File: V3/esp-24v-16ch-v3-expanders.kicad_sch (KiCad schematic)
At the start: 4 parts, among them U6 MCP23017_SS, U7 MCP23017_SS

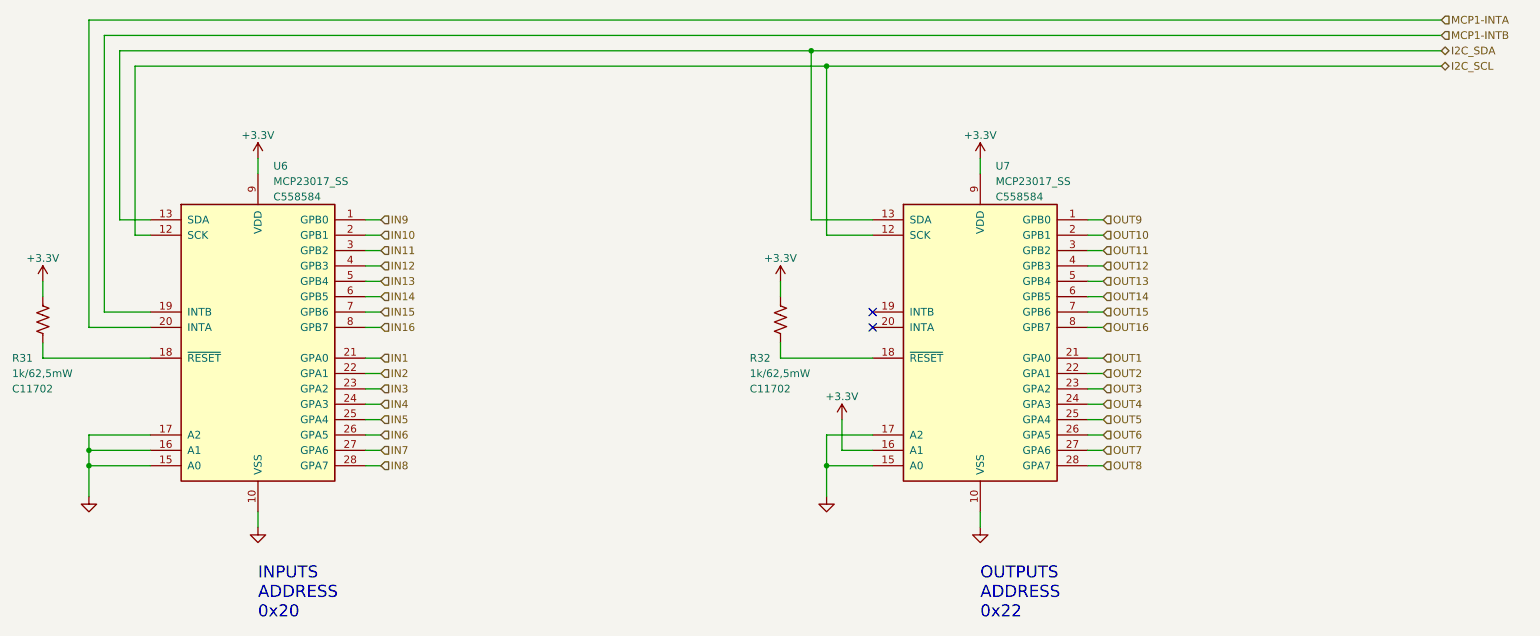
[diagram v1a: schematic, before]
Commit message: Added temperature sensor
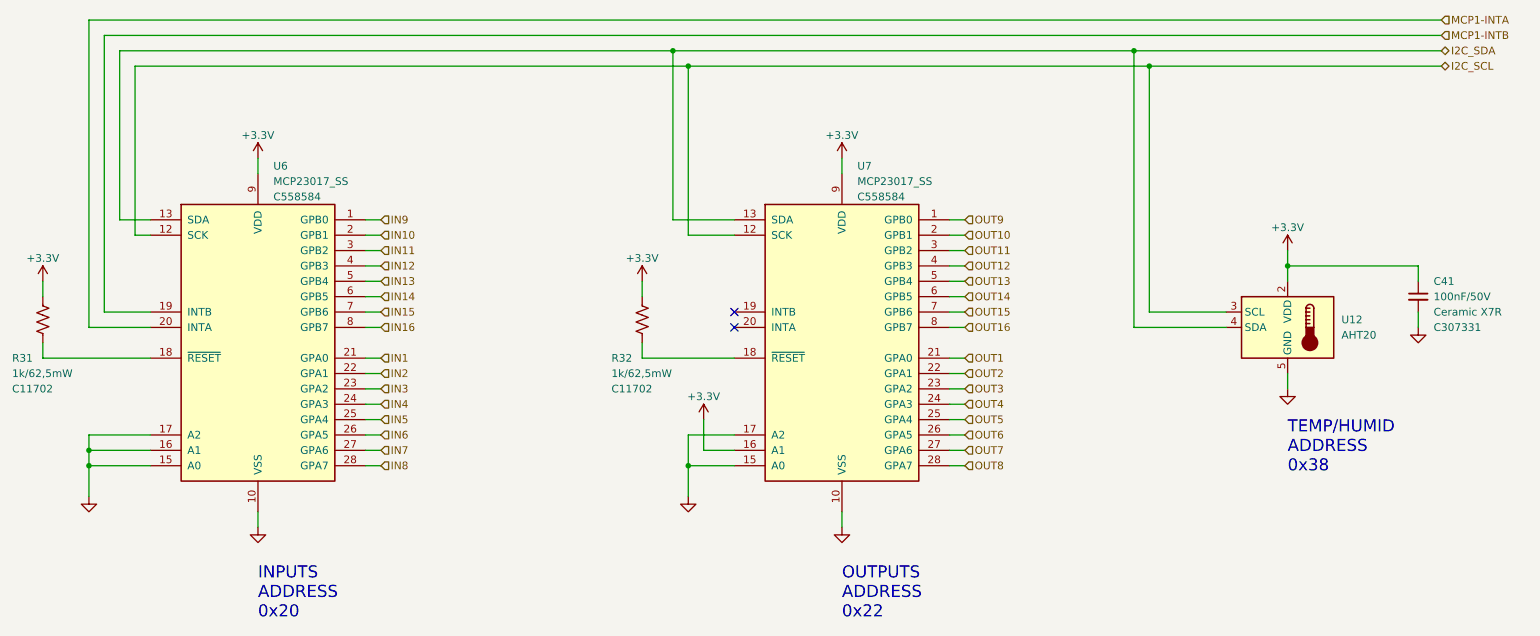
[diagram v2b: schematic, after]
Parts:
- added C41: 100nF/50V, Tales:C_0402_1005Metric, symbol Device:C_Small
- added U12: AHT20, Tales:DFN-6-3x3mm_P1mm, symbol Tales:AHT20
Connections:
- net +3.3V: now also C41.1, U12.2 (VDD)
- net GND: now also C41.2, U12.5 (GND)
- net I2C_SCL: now also U12.3 (SCL)
- net I2C_SDA: now also U12.4 (SDA)
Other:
- note added: "TEMP/HUMID ADDRESS 0x38"
- moved on the sheet: R32, U7

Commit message: Preparations for fabrication
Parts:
- U12: Case (none) -> DFN-6; JLCPCB BOM (none) -> 1; LCSC Part # (none) -> C2757850; Mfr (none) -> Aosong; Mfr PN (none) -> AHT20; Vendor (none) -> JLCPCB; Vendor PN (none) -> C2757850
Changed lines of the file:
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@@
+			)
+		)
+		(property "Case" "DFN-6"
+			(at 231.14 99.06 0)
+			(effects
+				(font
+					(size 1.27 1.27)
+				)
+				(hide yes)
+			)
+		)
+		(property "JLCPCB BOM" "1"
+			(at 231.14 99.06 0)
+			(effects
+				(font
+					(size 1.27 1.27)
+				)
+				(hide yes)
+			)
+		)
+		(property "LCSC Part #" "C2757850"
+			(at 231.14 99.06 0)
+			(effects
+				(font
+					(size 1.27 1.27)
+				)
+				(hide yes)
+			)
+		)
+		(property "Mfr" "Aosong"
+			(at 231.14 99.06 0)
+			(effects
+				(font
+					(size 1.27 1.27)
+				)
+				(hide yes)
+			)
+		)
+		(property "Mfr PN" "AHT20"
+			(at 231.14 99.06 0)
+			(effects
+				(font
+					(size 1.27 1.27)
+				)
+				(hide yes)
+			)
+		)
+		(property "Technology" "~"
+			(at 231.14 99.06 0)
+			(effects
+				(font
+					(size 1.27 1.27)
+				)
+				(hide yes)
+			)
+		)
+		(property "Vendor" "JLCPCB"
+			(at 231.14 99.06 0)
+			(effects
+				(font
+					(size 1.27 1.27)
+				)
+				(hide yes)
+			)
+		)
+		(property "Vendor PN" "C2757850"
+			(at 231.14 99.06 0)
+			(effects
+				(font
+					(size 1.27 1.27)
+				)
+				(hide yes)
 			)
 		)
